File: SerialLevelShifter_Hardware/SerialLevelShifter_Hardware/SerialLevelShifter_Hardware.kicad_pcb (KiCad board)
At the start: 2 copper layers, 11 parts, among them Q1 BSS138, Q2 BSS138, U1 AZ1117-3.3

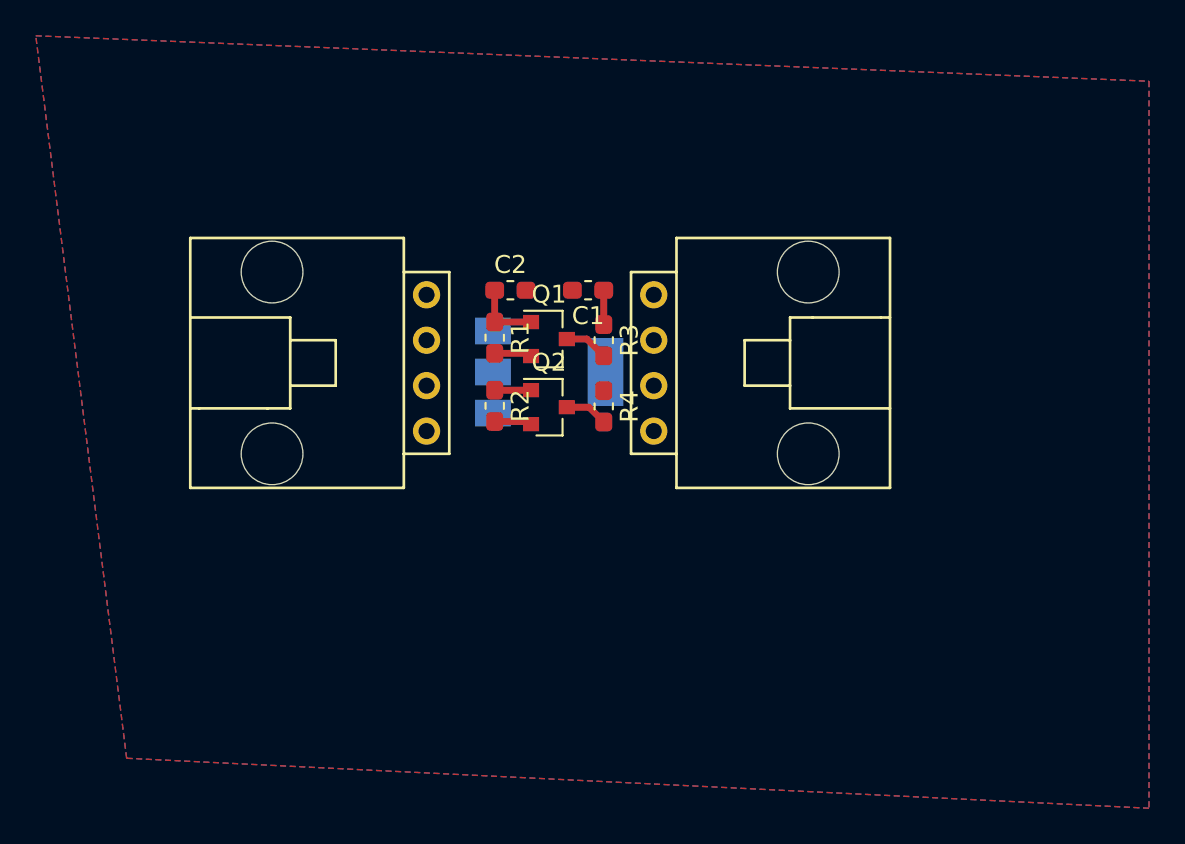
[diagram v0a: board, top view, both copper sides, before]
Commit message: finished layout
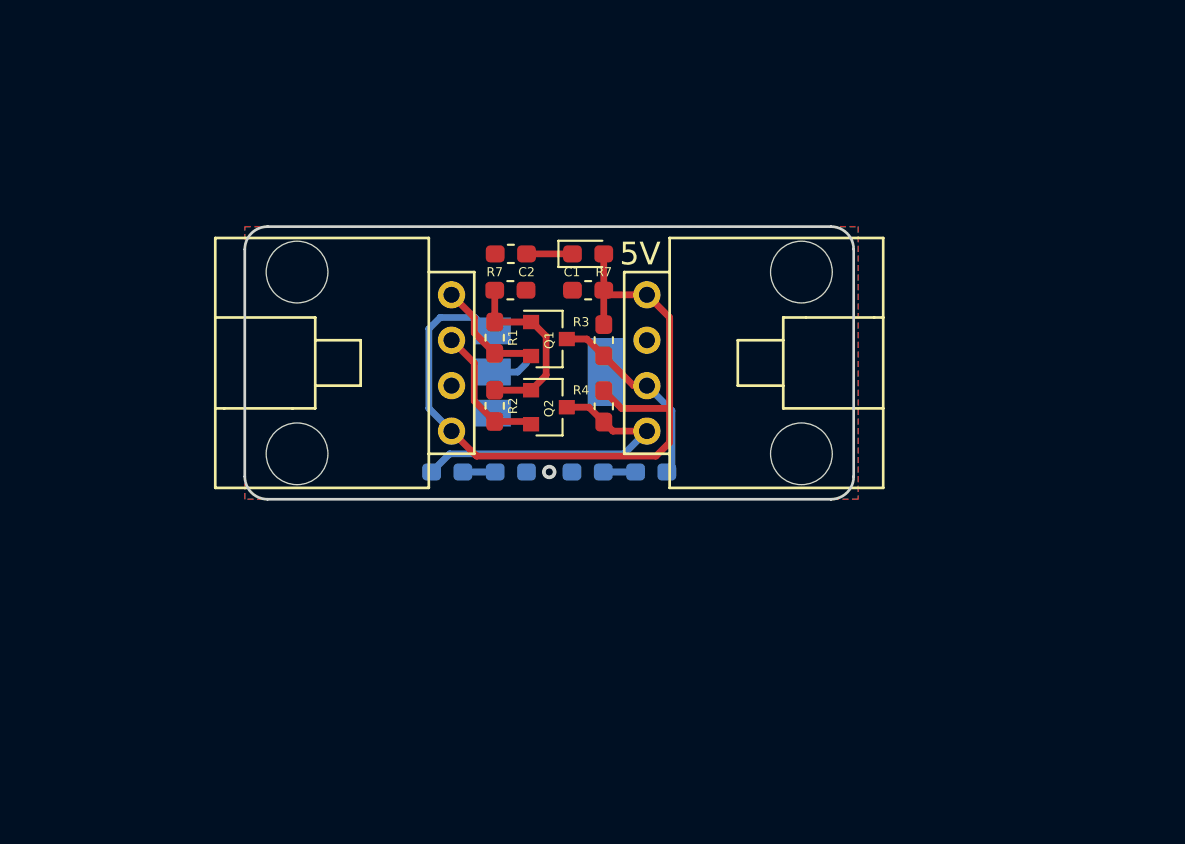
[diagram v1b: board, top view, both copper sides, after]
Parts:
- added D1: LED, LED_SMD:LED_0603_1608Metric_Pad1.05x0.95mm_HandSolder, B.Cu at (121.8, 68.3)
- added D2: LED, LED_SMD:LED_0603_1608Metric_Pad1.05x0.95mm_HandSolder, B.Cu at (110.4, 68.3)
- added R5: 500, Resistor_SMD:R_0603_1608Metric_Pad1.05x0.95mm_HandSolder, B.Cu at (118.2, 68.3)
- added R6: 500, Resistor_SMD:R_0603_1608Metric_Pad1.05x0.95mm_HandSolder, B.Cu at (113.9, 68.3)
- added R7: LED, LED_SMD:LED_0603_1608Metric_Pad1.05x0.95mm_HandSolder, F.Cu at (118.3, 56.1)
- added R7: 500, Resistor_SMD:R_0603_1608Metric_Pad1.05x0.95mm_HandSolder, F.Cu at (113.9, 56.1)
- moved Conn1 1.40 mm to (110.6, 66.0)
- moved Conn2 0.38 mm to (121.5, 58.4)
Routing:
- net +5V: track 1.92 -> 42.8 mm
- net 5V_Rx: track 2.41 -> 18.0 mm
- net 5V_Tx: track 2.45 -> 11.1 mm
- net +3V3: track 5.84 -> 12.5 mm
- net 3V3_Tx: track 2.09 -> 7.64 mm
- net 3V3_Rx: track 2.09 -> 6.37 mm
- net Net-(D3-Pad1): track 0.00 -> 2.57 mm
- net Net-(D2-Pad1): track 0.00 -> 1.81 mm
- net Net-(D1-Pad1): track 0.00 -> 1.81 mm
- net GND: vias 0 -> 1
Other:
- board outline added: 34 x 15.2 mm
- board text added: "+5V"
- board text added: "3V3"
- board text added: "5V"
- board text added: "GND"
- board text added: "Rx"
- board text added: "Tx"
